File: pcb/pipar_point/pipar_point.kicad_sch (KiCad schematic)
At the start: 83 parts, among them Q1 AO3416 N-channel MOSFET, SW1 SW_Wuerth_450301014042, SW2 CK_KMS2xxG, U1 Seeeduino Xiao nRF52840, U2 74HC595

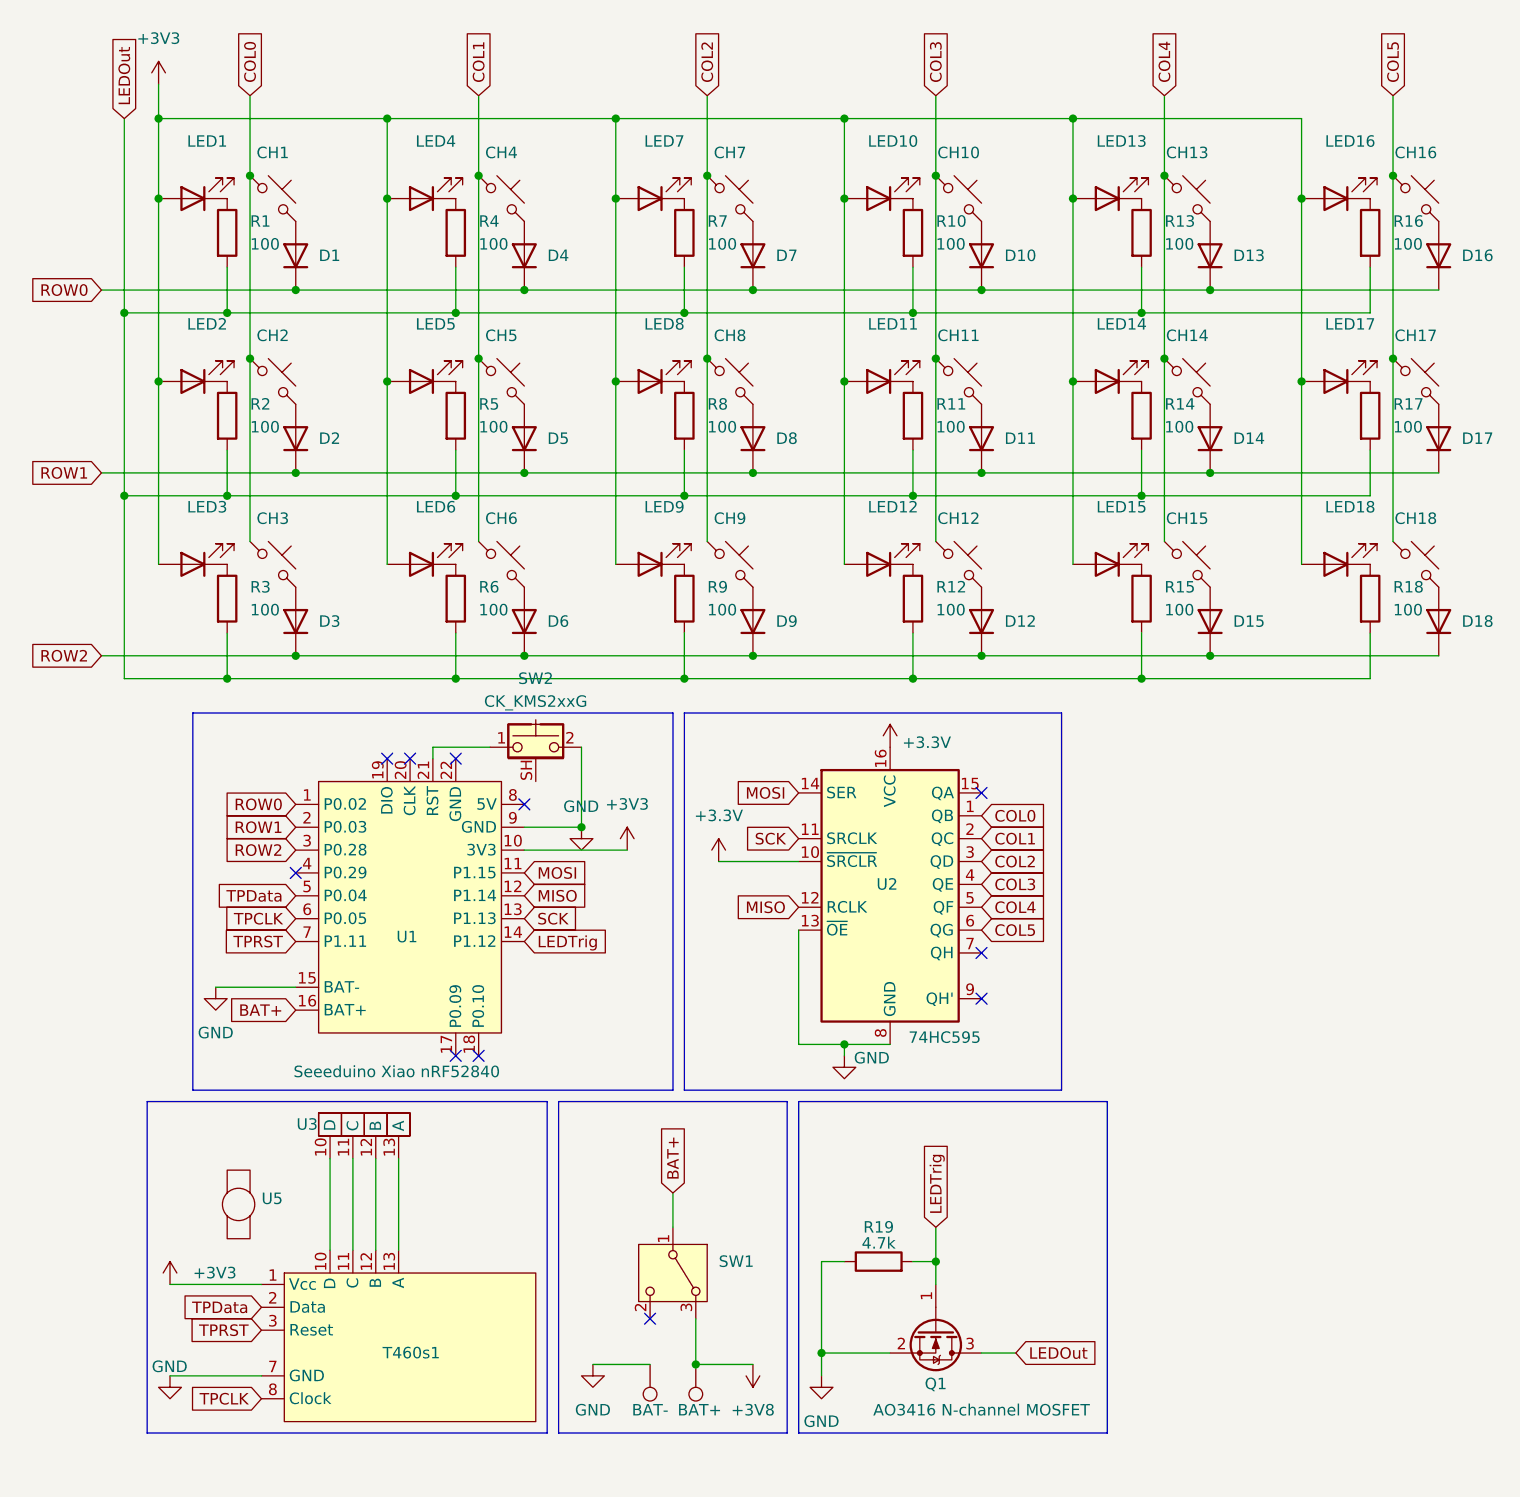
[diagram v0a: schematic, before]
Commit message: Finish setting up the board
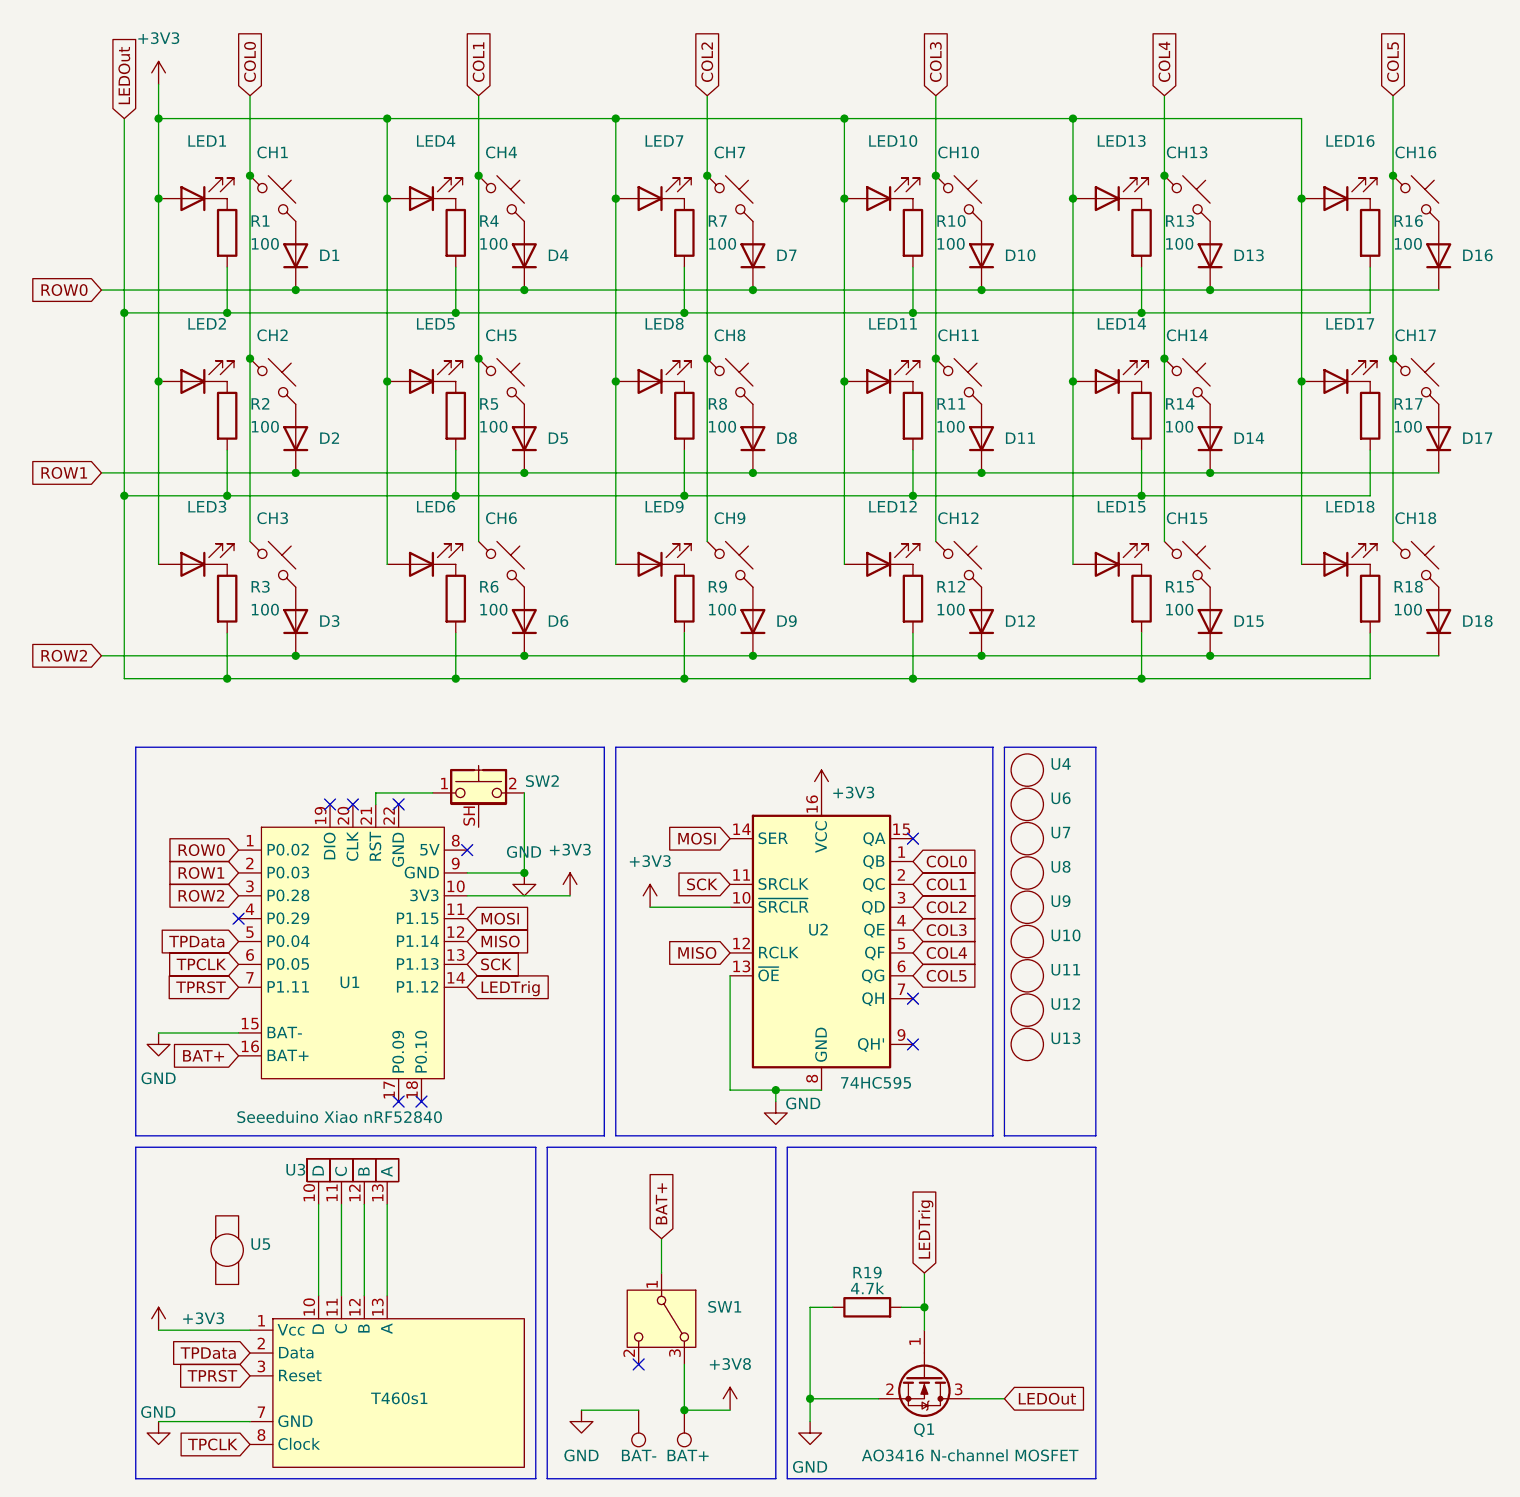
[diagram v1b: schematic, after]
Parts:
- added U10, U11, U12, U13, U4, U6, U8, U9: ~, choc:Solder Nut, symbol Trackpoint:Solder_Nut
- added U7: ~, Art:Salt, symbol Trackpoint:Solder_Nut
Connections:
- net +3.3V is gone; now on net +3V3: U2.10 (~{SRCLR}), U2.16 (VCC)
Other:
- moved on the sheet: Q1, R19, SW1, SW2, T460s1, U1, U2, U3, U5
